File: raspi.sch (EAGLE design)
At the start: 5 parts

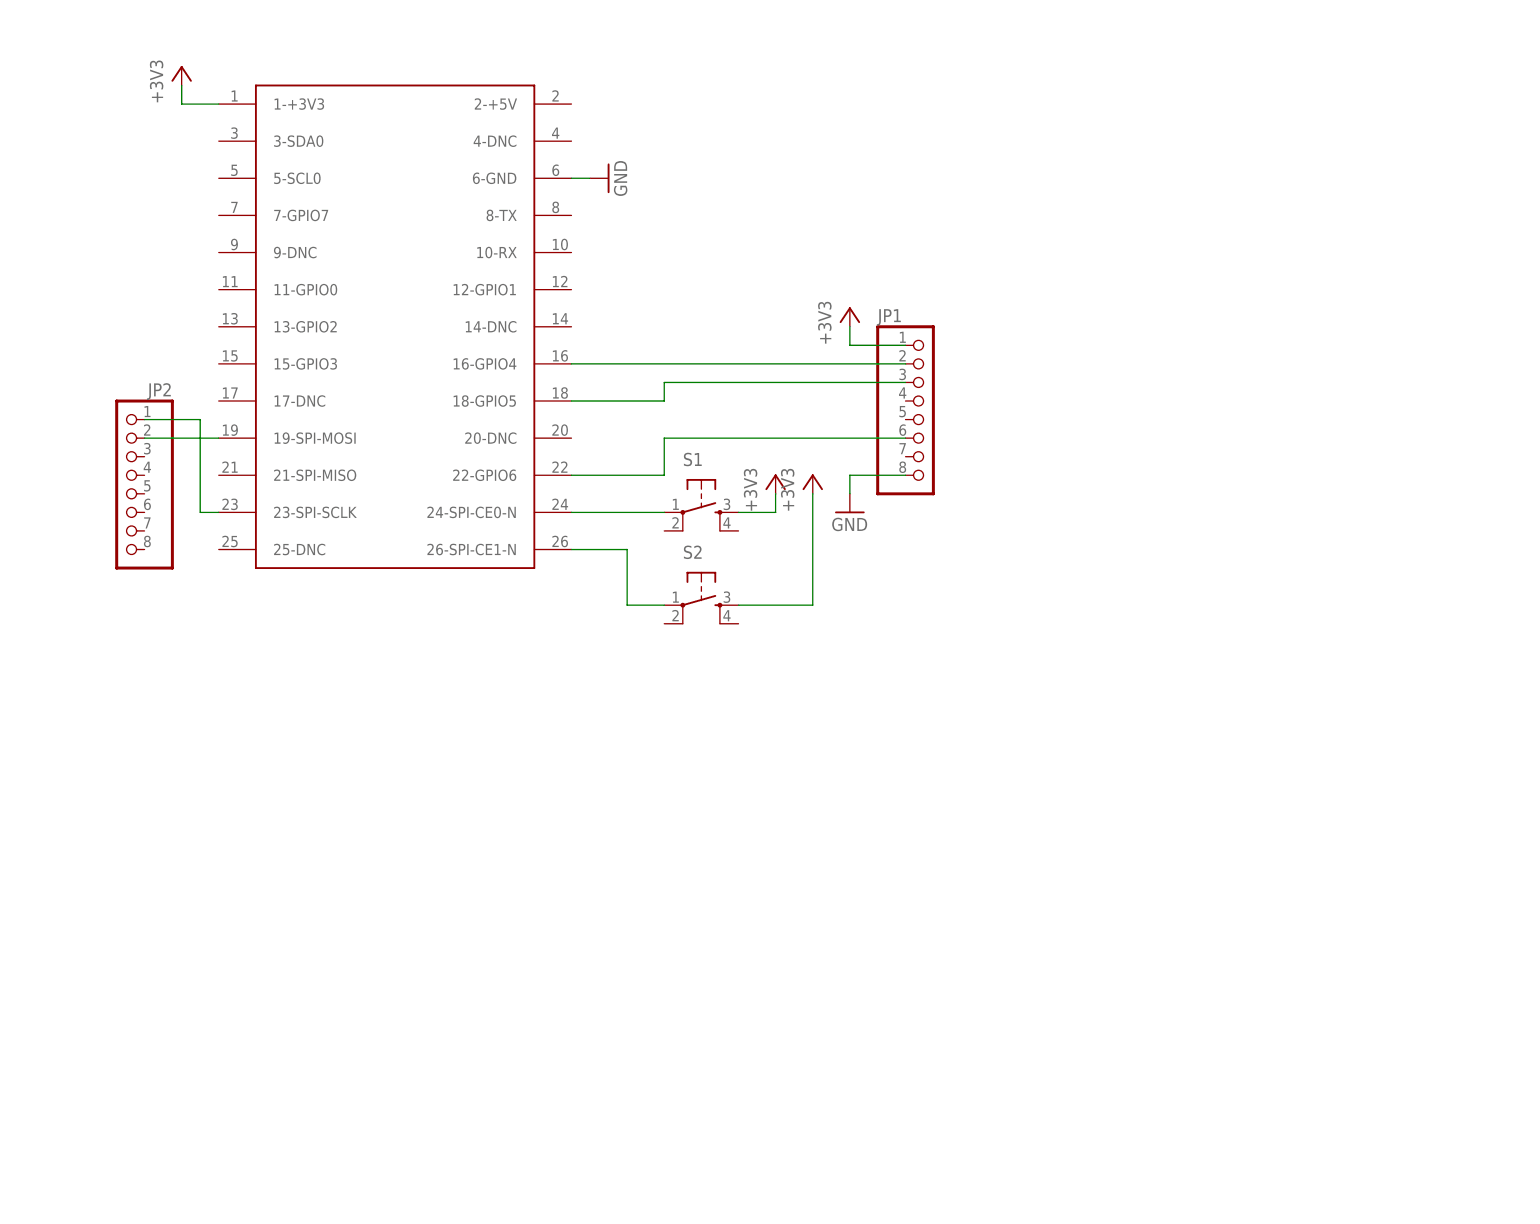
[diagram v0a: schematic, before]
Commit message: work on shield
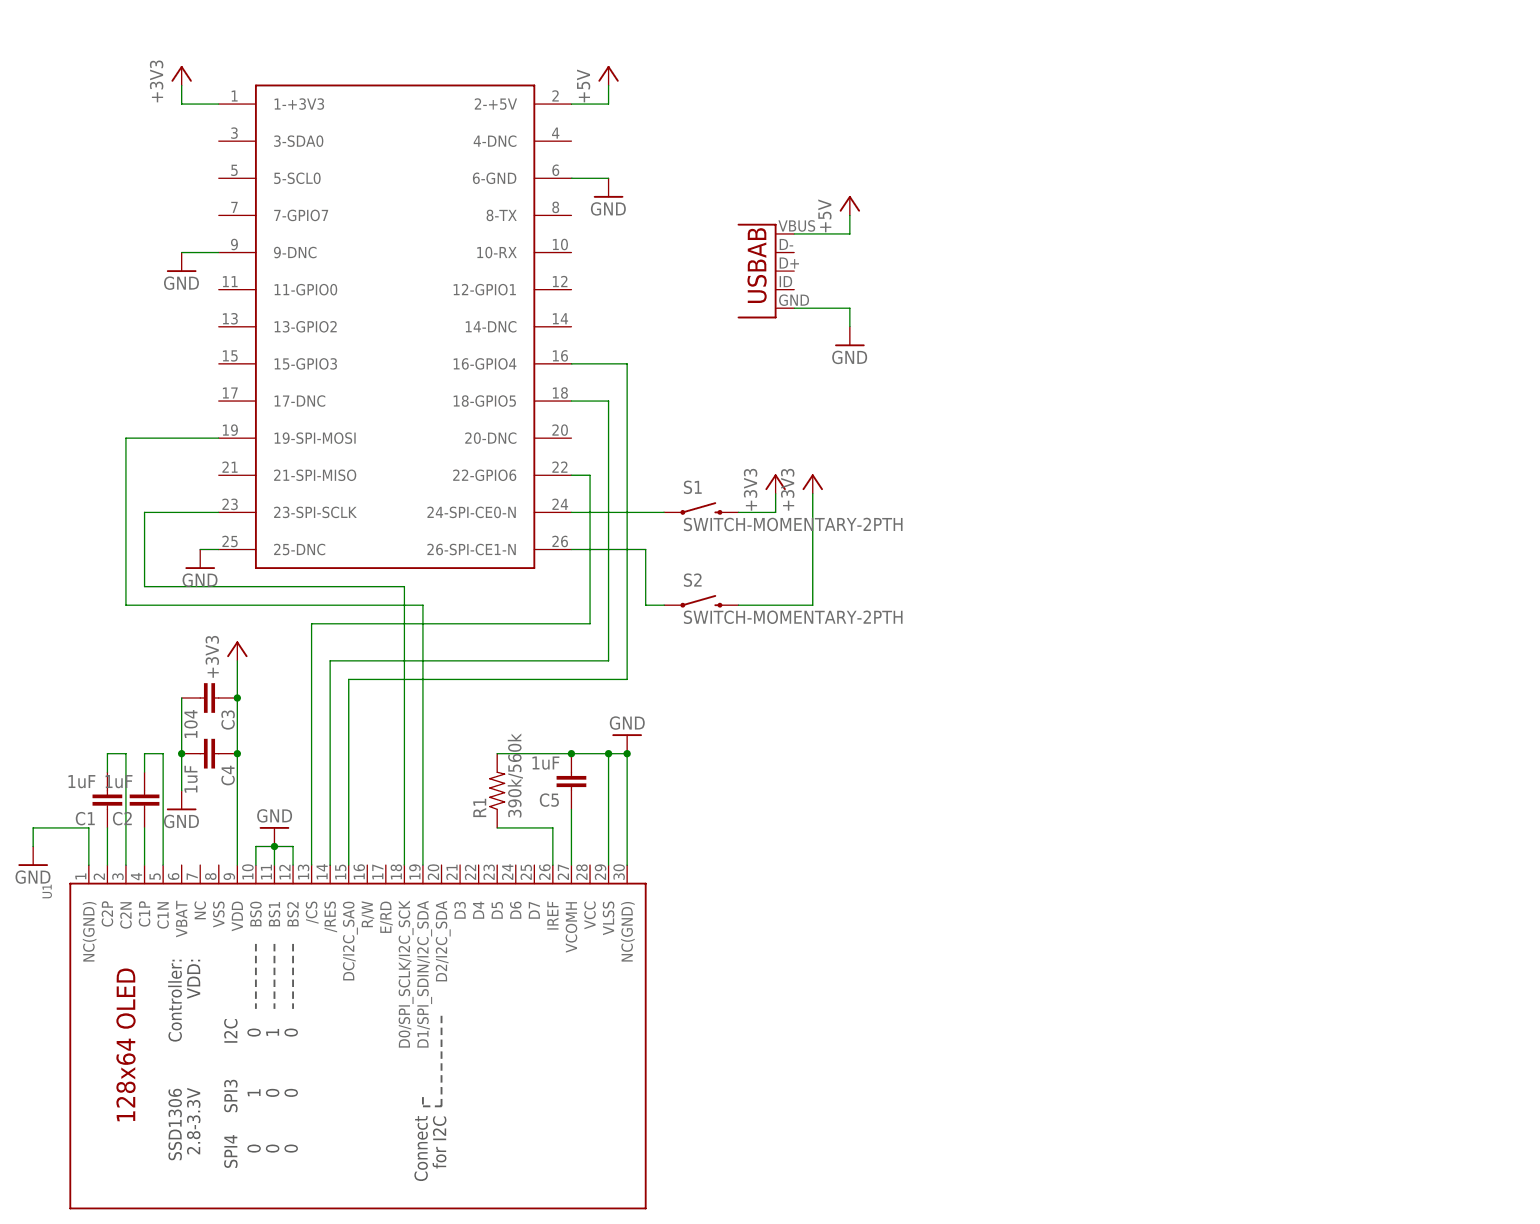
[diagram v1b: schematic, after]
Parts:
- removed JP1, JP2: (no value), pinhead:PINHD-1X8
- added C1, C2, C4, C5: 1uF, SparkFun-Capacitors:CAP0805
- added C3: 104, SparkFun-Capacitors:CAP0805
- added R1: 390k/560k, SparkFun-Resistors:RESISTOR0805-RES
- added U$2: USB_AB, SparkFun-Connectors:USB_AB
- added U1: (no value), microbuilder:DISP_OLED_UG-2864HSWEG010.96"
- S1, S2: value (none) -> SWITCH-MOMENTARY-2PTH; device SparkFun:TAC_SWITCHPTH -> SparkFun-Electromechanical:SWITCH-MOMENTARY-2PTH
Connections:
- new net +5V: U$1.2-+5V, U$2.VBUS
- new net N$1: U$1.19-SPI-MOSI, U1.D1/SPI_SDIN/I2C_SDA
- new net N$10: C1.1, U1.C2P
- new net N$11: C2.1, U1.C1P
- new net N$12: C1.2, U1.C2N
- new net N$13: C2.2, U1.C1N
- new net N$4: U$1.16-GPIO4, U1.DC/I2C_SA0
- net +3V3: now also C3.1, C4.1, S1.2, S2.2, U1.VDD; no longer JP1.1, S1.3, S2.3
- net GND: now also C3.2, C4.2, C5.2, R1.2, U$1.25-DNC, U$1.9-DNC, U$2.GND, U1.BS0, U1.BS1, U1.BS2, U1.NC(GND)@1, U1.NC(GND)@2, U1.VLSS; no longer JP1.8
- net N$5: now also U1.D0/SPI_SCLK/I2C_SCK; no longer JP2.1
- net N$6: now also C5.1, U1.VCOMH; no longer JP2.2, U$1.19-SPI-MOSI
- net N$7: now also U1./CS; no longer JP1.6
- net N$8: now also U1./RES; no longer JP1.3
- net N$9: now also R1.1, U1.IREF; no longer JP1.2, U$1.16-GPIO4

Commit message: work in progress
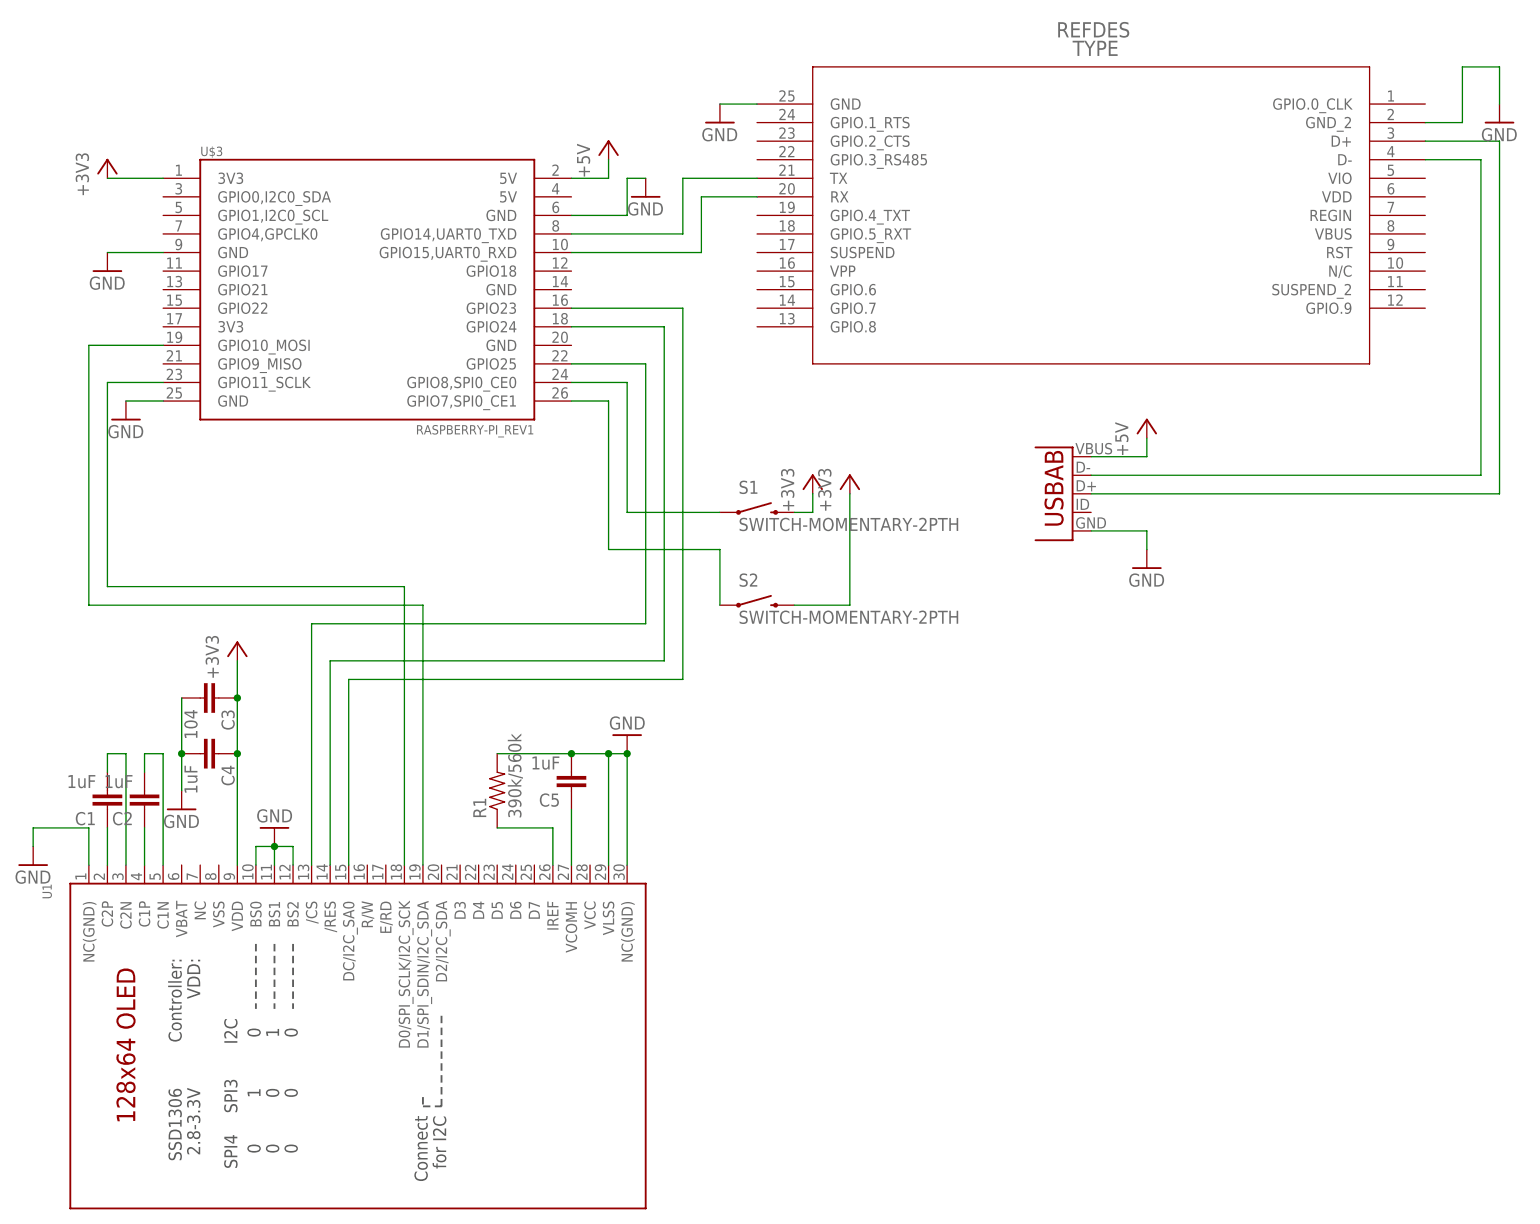
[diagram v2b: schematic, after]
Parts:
- removed U$1: RASPBERRY-PI, RaspberryPi:RASPBERRY-PI
- added U$3: RASPBERRY-PI_REV1, RaspberryPi:RASPBERRY-PI_REV1
- added U2: CP2110-F01-GM, bxl_import:CP2110-F01-GM
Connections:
- new net N$14: U$2.D-, U2.D-
- new net N$15: U$2.D+, U2.D+
- new net N$16: U$3.GPIO14,UART0_TXD, U2.TX
- new net N$17: U$3.GPIO15,UART0_RXD, U2.RX
- net +3V3: now also U$3.3V3@1; no longer U$1.1-+3V3
- net +5V: now also U$3.5V@2; no longer U$1.2-+5V
- net GND: now also U$3.GND@25, U$3.GND@6, U$3.GND@9, U2.GND, U2.GND_2; no longer U$1.25-DNC, U$1.6-GND, U$1.9-DNC
- net N$1: now also U$3.GPIO10_MOSI; no longer U$1.19-SPI-MOSI
- net N$2: now also U$3.GPIO7,SPI0_CE1; no longer U$1.26-SPI-CE1-N
- net N$3: now also U$3.GPIO8,SPI0_CE0; no longer U$1.24-SPI-CE0-N
- net N$4: now also U$3.GPIO23; no longer U$1.16-GPIO4
- net N$5: now also U$3.GPIO11_SCLK; no longer U$1.23-SPI-SCLK
- net N$7: now also U$3.GPIO25; no longer U$1.22-GPIO6
- net N$8: now also U$3.GPIO24; no longer U$1.18-GPIO5
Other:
- moved on the sheet: S1, S2
